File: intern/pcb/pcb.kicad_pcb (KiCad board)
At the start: 2 copper layers, 99.5 x 76 mm, 33 parts, among them J1 Conn_01x02, J10 Conn_01x04, J11 Conn_01x04, J12 RJ45, J13 Screw_Terminal_01x04, J14 Screw_Terminal_01x04, J15 Screw_Terminal_01x04, J16 Conn_01x04, J2 Conn_01x02, J3 Conn_01x02, J4 Conn_01x02, J5 Conn_01x02, J6 Conn_01x02, J7 Conn_01x02, J8 Conn_01x02, J9 Conn_01x02, U2 STM32F103C8T6, U5 TPS54360DDA, U6 LM1117-3.3

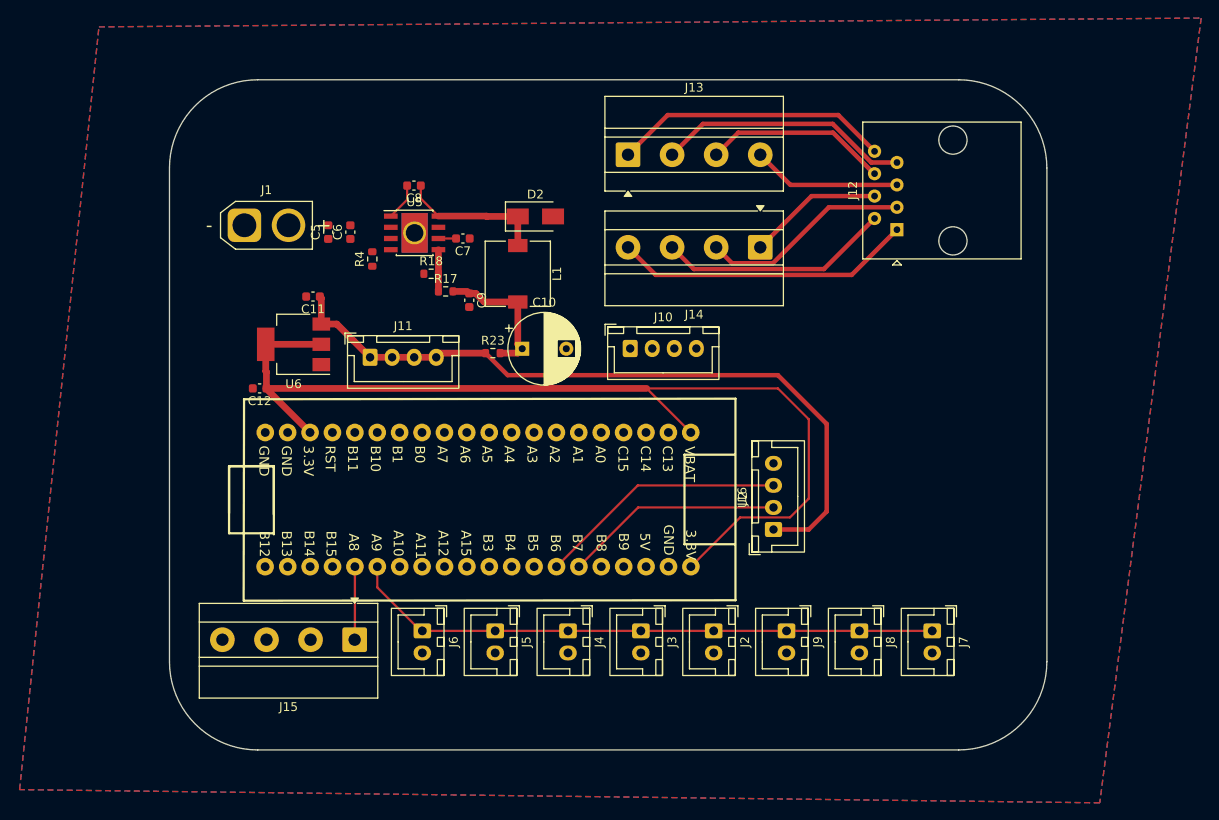
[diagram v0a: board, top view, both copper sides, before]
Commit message: finalize intern pcb with gbr
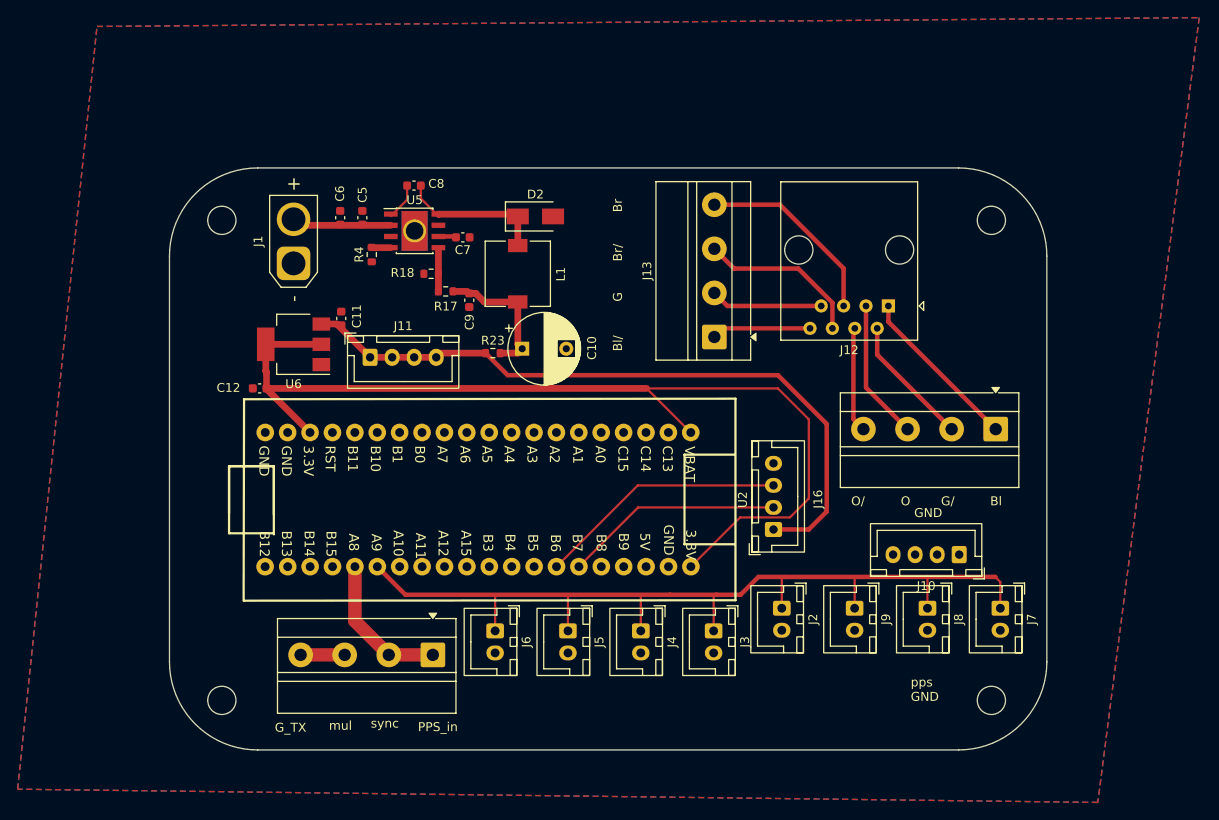
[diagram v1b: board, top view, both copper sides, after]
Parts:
- added H1: MountingHole, HKUST_RDC2025_Footprint_Lib:MountingHole_3.2mm_M3, F.Cu at (66.4, 182.4)
- added H2: MountingHole, HKUST_RDC2025_Footprint_Lib:MountingHole_3.2mm_M3, F.Cu at (153.7, 127.9)
- added H3: MountingHole, HKUST_RDC2025_Footprint_Lib:MountingHole_3.2mm_M3, F.Cu at (66.4, 127.9)
- added H4: MountingHole, HKUST_RDC2025_Footprint_Lib:MountingHole_3.2mm_M3, F.Cu at (153.7, 182.4)
- moved J10 44.0 mm to (150.1, 165.8), turned to 180 degrees
- moved J14 33.7 mm to (154.2, 151.6)
- moved J13 22.9 mm to (122.3, 141.2), turned to 90 degrees
- moved J15 9.04 mm to (90.4, 177.2)
- moved J12 8.70 mm to (142.0, 137.7), turned to 180 degrees
- moved J4 8.26 mm to (114.0, 174.5)
- moved J6 8.26 mm to (97.4, 174.5)
- moved J3 8.25 mm to (122.2, 174.5)
- moved J5 8.25 mm to (105.7, 174.5)
- moved J8 8.14 mm to (146.5, 171.9)
- moved J9 8.14 mm to (138.2, 171.9)
- moved J2 8.14 mm to (129.9, 171.9)
- moved J7 8.14 mm to (154.7, 171.9)
- moved J1 7.05 mm to (74.6, 132.8), turned to 90 degrees
- moved C5 4.20 mm to (82.4, 127.6), turned to -90 degrees
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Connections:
- J14 pad 1: /Bl -> /O/
- J14 pad 2: /G/ -> /O
- J14 pad 3: /O -> /G/
- J14 pad 4: /O/ -> /Bl
- J15 pad 2: unconnected-(J15-Pin_2-Pad2) -> /pps_in
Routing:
- net /pps: track 67.3 -> 103.3 mm
- net /Br: track 31.5 -> 11.3 mm
- net /Br/: track 28.8 -> 12.7 mm
- net /O/: track 33.9 -> 19.0 mm
- net +24V: track 0.00 -> 11.6 mm
- net /O: track 26.4 -> 14.9 mm
- net /pps_in: track 8.30 -> 16.6 mm
- net /G/: track 23.9 -> 15.9 mm
- net /gnss_TX: track 0.00 -> 5.00 mm
- net /Bl/: track 16.9 -> 21.9 mm
- net /Bl: track 15.4 -> 12.0 mm
- net +5V: track 82.4 -> 79.2 mm
- net Net-(U5-RT/CLK): track 0.00 -> 2.18 mm
- net /G: track 20.9 -> 18.8 mm
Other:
- board size 99.5 x 76 mm -> 99.5 x 66 mm
- board text added: "Bl"
- board text added: "Bl/"
- board text added: "Br"
- board text added: "Br/"
- board text added: "G"
- board text added: "G/"
- board text added: "GND"
- board text added: "G_TX"
- board text added: "O"
- board text added: "O/"
- board text added: "PPS_in"
- board text added: "mul"
- board text added: "pps GND"
- board text added: "sync"
